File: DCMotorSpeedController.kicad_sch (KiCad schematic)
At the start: 15 parts, among them J1 Motor Terminal, J2 Power Terminal, Q1 IRLZ44N, SW1 POWER_SW, U1 NE555P

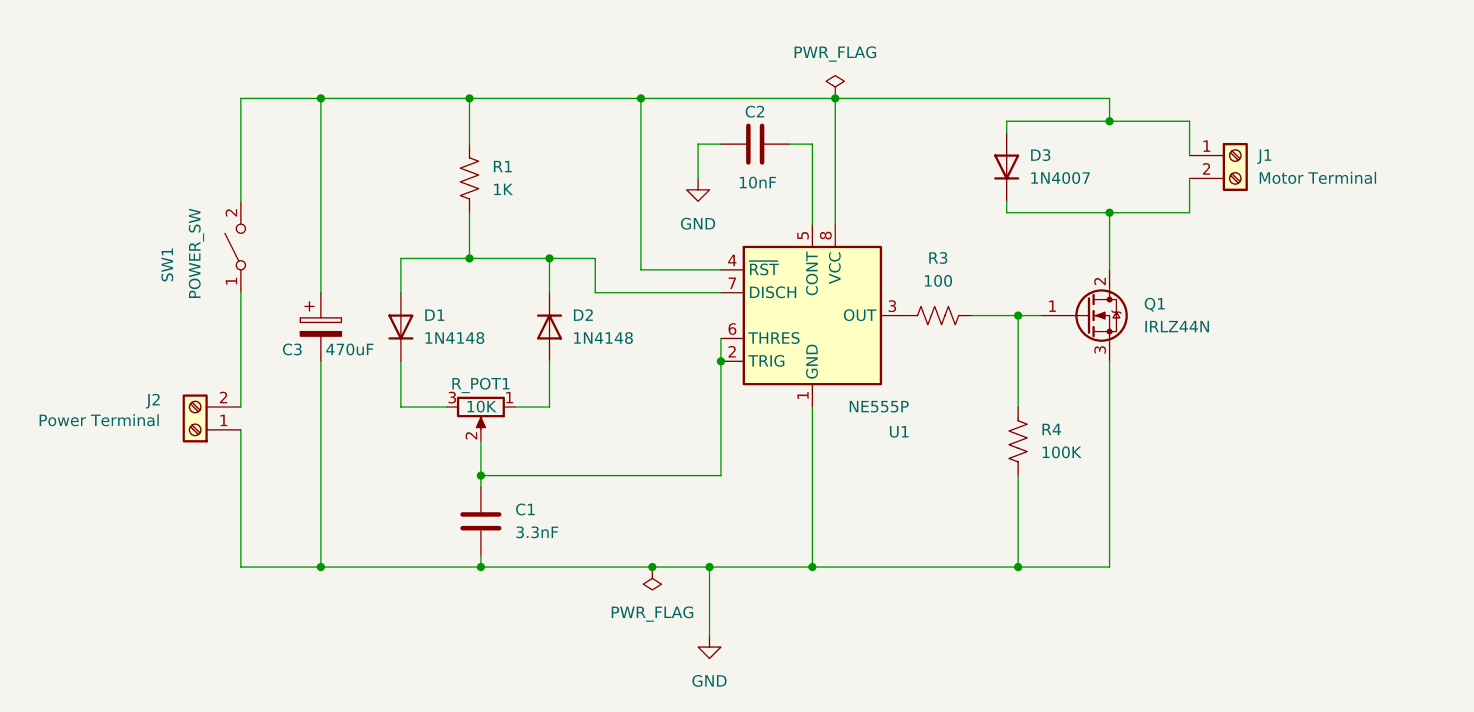
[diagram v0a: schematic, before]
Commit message: more stuff
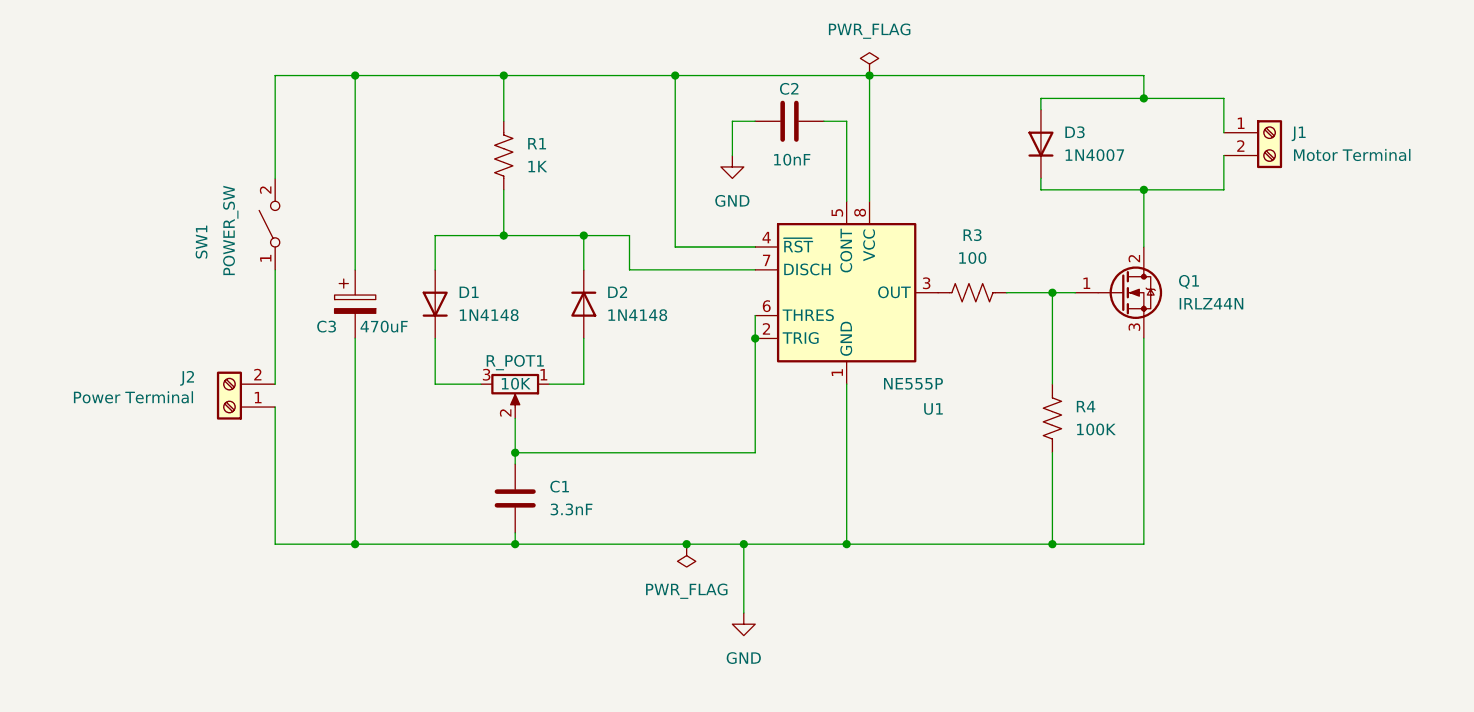
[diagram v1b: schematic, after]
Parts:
- C1, C2, C3: KiLib_Generator (none) -> capacitor/THT/other
- D1, D2, D3: KiLib_Generator (none) -> diode/THT
- J1, J2: KiLib_Generator (none) -> terminal_block/MaiXu
- Q1: KiLib_Generator (none) -> package/TO_SOT/THT
- R1, R3, R4: KiLib_Generator (none) -> resistor/THT
- U1: KiLib_Generator (none) -> package/DIP/legacy
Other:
- moved on the sheet: C1, C2, C3, D1, D2, D3, J1, J2, Q1, R1, R3, R4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
